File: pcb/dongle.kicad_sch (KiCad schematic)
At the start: 32 parts, among them J1 USB_A, J2 Conn_01x01_Pin, J3 Conn_01x01_Pin, J4 Conn_01x01_Pin, J5 Conn_01x01_Pin, SW1 SW_Push_45deg, U3 nRF52833_QDxx, Y1 32MHz

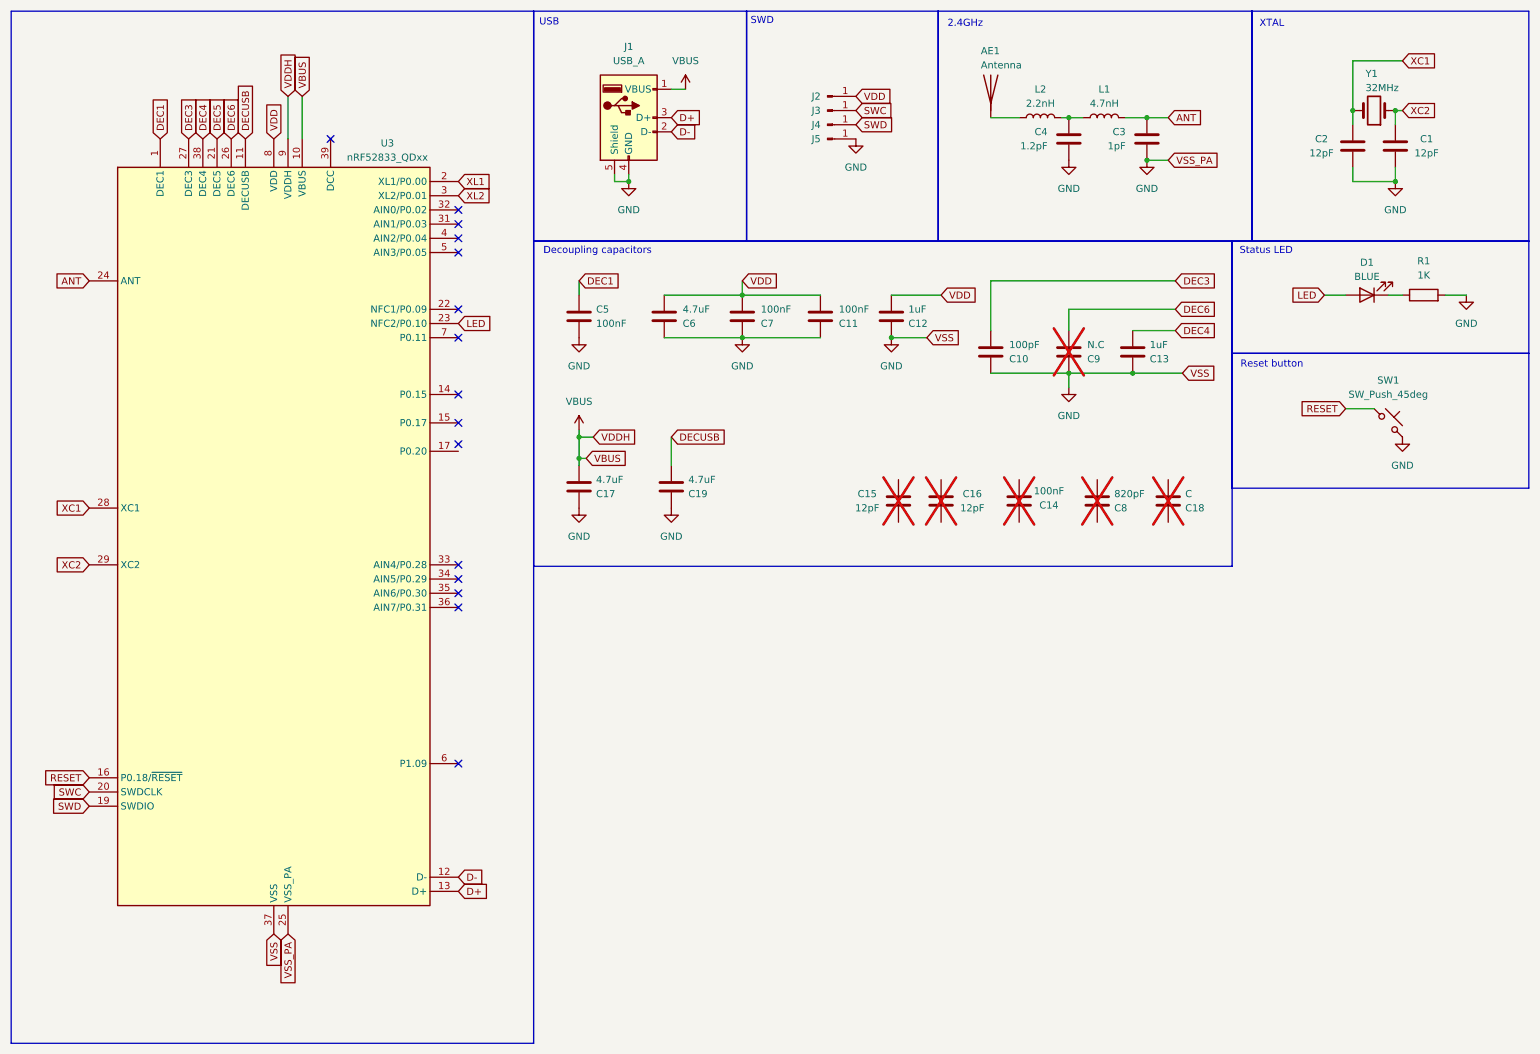
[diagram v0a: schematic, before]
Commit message: update pcb
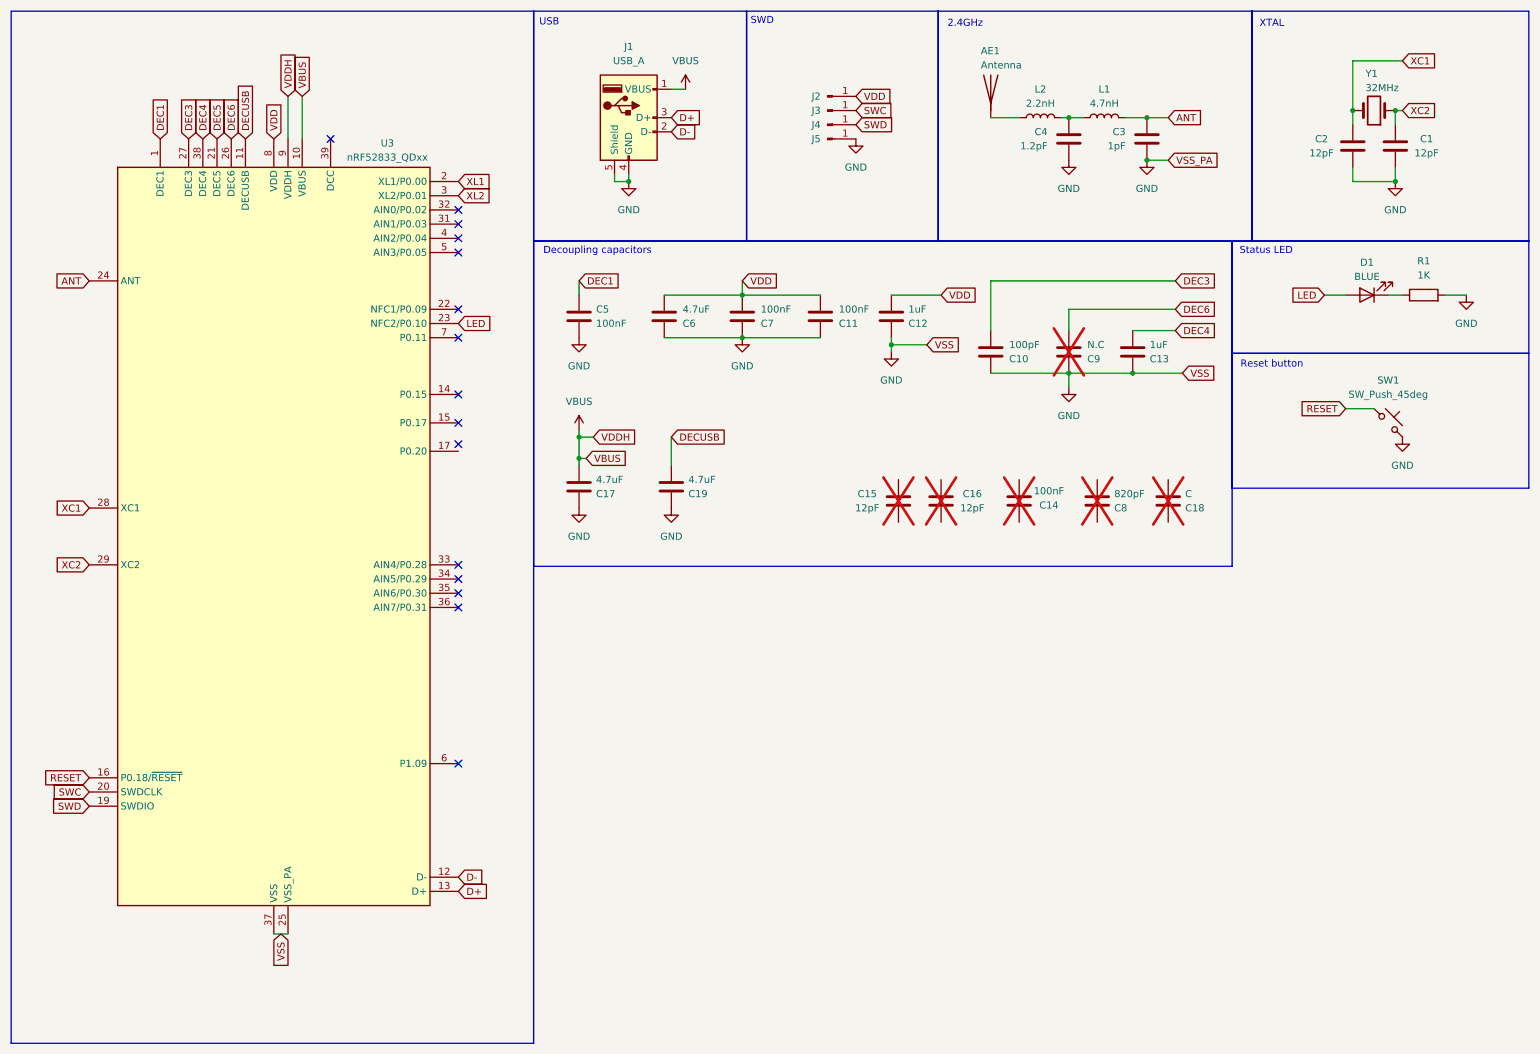
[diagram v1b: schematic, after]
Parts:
- AE1: footprint (none) -> dongle:Texas_SWRA117D_2.4GHz_Left
- D1: footprint (none) -> dongle:LED_0603_1608Metric
- R1: footprint (none) -> dongle:R_0201_0603Metric_Pad0.64x0.40mm_HandSolder
- SW1: footprint (none) -> dongle:TS342A2P
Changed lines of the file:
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@@
 	)
 	(junction
+		(at 170.18 72.39)
+		(diameter 0)
+		(color 0 0 0 0)
+	)
+	(junction
 		(at 201.93 31.75)
 		(diameter 0)
@@
 	)
 	(junction
-		(at 170.18 71.12)
-		(diameter 0)
-		(color 0 0 0 0)
-	)
-	(junction
 		(at 114.3 92.71)
 		(diameter 0)
@@
 	(wire
 		(pts
+			(xy 170.18 72.39) (xy 170.18 73.66)
+		)
+		(stroke
+			(width 0)
+			(type default)
+		)
+	)
+	(wire
+		(pts
 			(xy 220.98 60.96) (xy 187.96 60.96)
 		)
@@
 	(wire
 		(pts
+			(xy 170.18 71.12) (xy 170.18 72.39)
+		)
+		(stroke
+			(width 0)
+			(type default)
+		)
+	)
+	(wire
+		(pts
 			(xy 219.71 39.37) (xy 215.9 39.37)
 		)
@@
 	(wire
 		(pts
+			(xy 176.53 72.39) (xy 170.18 72.39)
+		)
+		(stroke
+			(width 0)
+			(type default)
+		)
+	)
+	(wire
+		(pts
 			(xy 251.46 63.5) (xy 247.65 63.5)
 		)
@@
 	(wire
 		(pts
-			(xy 273.05 63.5) (xy 269.24 63.5)
+			(xy 59.69 177.8) (xy 62.23 177.8)
 		)
 		(stroke
@@
 	(wire
 		(pts
-			(xy 252.73 21.59) (xy 252.73 30.48)
+			(xy 273.05 63.5) (xy 269.24 63.5)
 		)
 		(stroke
@@
 	(wire
 		(pts
-			(xy 176.53 71.12) (xy 170.18 71.12)
+			(xy 252.73 21.59) (xy 252.73 30.48)
 		)
 		(stroke
@@
 		)
 	)
-	(global_label "VSS"
+	(global_label "D+"
 		(shape input)
-		(at 176.53 71.12 0)
+		(at 130.81 31.75 0)
 		(fields_autoplaced yes)
 		(effects
@@
 		)
 		(property "Intersheetrefs" "${INTERSHEET_REFS}"
-			(at 183.0228 71.12 0)
+			(at 136.6376 31.75 0)
 			(effects
 				(font
@@
 		)
 	)
-	(global_label "D+"
+	(global_label "DEC5"
 		(shape input)
-		(at 130.81 31.75 0)
+		(at 49.53 35.56 90)
 		(fields_autoplaced yes)
 		(effects
@@
 		)
 		(property "Intersheetrefs" "${INTERSHEET_REFS}"
-			(at 136.6376 31.75 0)
+			(at 49.53 27.6763 90)
 			(effects
 				(font
@@
 		)
 	)
-	(global_label "DEC5"
+	(global_label "DEC1"
 		(shape input)
-		(at 49.53 35.56 90)
+		(at 39.37 35.56 90)
 		(fields_autoplaced yes)
 		(effects
@@
 		)
 		(property "Intersheetrefs" "${INTERSHEET_REFS}"
-			(at 49.53 27.6763 90)
+			(at 39.37 27.6763 90)
 			(effects
 				(font
@@
 		)
 	)
-	(global_label "DEC1"
+	(global_label "ANT"
 		(shape input)
-		(at 39.37 35.56 90)
+		(at 219.71 31.75 0)
 		(fields_autoplaced yes)
 		(effects
@@
 		)
 		(property "Intersheetrefs" "${INTERSHEET_REFS}"
-			(at 39.37 27.6763 90)
+			(at 226.0819 31.75 0)
 			(effects
 				(font
@@
 		)
 	)
-	(global_label "ANT"
+	(global_label "VDD"
 		(shape input)
-		(at 219.71 31.75 0)
+		(at 59.69 35.56 90)
 		(fields_autoplaced yes)
 		(effects
@@
 		)
 		(property "Intersheetrefs" "${INTERSHEET_REFS}"
-			(at 226.0819 31.75 0)
+			(at 59.69 28.9462 90)
 			(effects
 				(font
@@
 		)
 	)
-	(global_label "VDD"
+	(global_label "VSS"
 		(shape input)
-		(at 59.69 35.56 90)
+		(at 176.53 72.39 0)
 		(fields_autoplaced yes)
 		(effects
@@
 		)
 		(property "Intersheetrefs" "${INTERSHEET_REFS}"
-			(at 59.69 28.9462 90)
+			(at 183.0228 72.39 0)
 			(effects
 				(font
@@
 		)
 	)
-	(global_label "VSS"
-		(shape input)
-		(at 59.69 177.8 270)
-		(fields_autoplaced yes)
-		(effects
-			(font
-				(size 1.27 1.27)
-			)
-			(justify right)
-		)
-		(property "Intersheetrefs" "${INTERSHEET_REFS}"
-			(at 59.69 184.2928 90)
-			(effects
-				(font
-					(size 1.27 1.27)
-				)
-				(justify right)
-				(hide yes)
-			)
-		)
-	)
 	(global_label "DEC1"
 		(shape input)
@@
 		)
 	)
+	(global_label "VSS"
+		(shape input)
+		(at 60.96 177.8 270)
+		(fields_autoplaced yes)
+		(effects
+			(font
+				(size 1.27 1.27)
+			)
+			(justify right)
+		)
+		(property "Intersheetrefs" "${INTERSHEET_REFS}"
+			(at 60.96 184.2928 90)
+			(effects
+				(font
+					(size 1.27 1.27)
+				)
+				(justify right)
+				(hide yes)
+			)
+		)
+	)
 	(global_label "VDD"
 		(shape input)
@@
 		)
 	)
-	(global_label "VSS_PA"
-		(shape input)
-		(at 62.23 177.8 270)
-		(fields_autoplaced yes)
-		(effects
-			(font
-				(size 1.27 1.27)
-			)
-			(justify right)
-		)
-		(property "Intersheetrefs" "${INTERSHEET_REFS}"
-			(at 62.23 187.619 90)
-			(effects
-				(font
-					(size 1.27 1.27)
-				)
-				(justify right)
-				(hide yes)
-			)
-		)
-	)
 	(global_label "DEC6"
 		(shape input)
@@
 			)
 		)
-		(property "Footprint" ""
+		(property "Footprint" "dongle:TS342A2P"
 			(at 259.08 86.36 0)
 			(effects
@@
 	(symbol
 		(lib_id "Library:GND")
-		(at 170.18 71.12 0)
+		(at 170.18 73.66 0)
 		(unit 1)
 		(exclude_from_sim no)
@@
 		(fields_autoplaced yes)
 		(property "Reference" "#PWR07"
-			(at 170.18 77.47 0)
+			(at 170.18 80.01 0)
 			(effects
 				(font
@@
 		)
 		(property "Value" "GND"
-			(at 170.18 76.2 0)
+			(at 170.18 78.74 0)
 			(effects
 				(font
@@
 		)
 		(property "Footprint" ""
-			(at 170.18 71.12 0)
+			(at 170.18 73.66 0)
 			(effects
 				(font
@@
 		)
 		(property "Datasheet" ""
-			(at 170.18 71.12 0)
+			(at 170.18 73.66 0)
 			(effects
 				(font
@@
 		)
 		(property "Description" "Global ground symbol"
-			(at 170.18 80.518 0)
+			(at 170.18 83.058 0)
 			(effects
 				(font
@@
 			)
 		)
-		(property "Footprint" ""
+		(property "Footprint" "dongle:Texas_SWRA117D_2.4GHz_Left"
 			(at 187.96 26.67 0)
 			(effects
@@
 			)
 		)
-		(property "Footprint" ""
+		(property "Footprint" "dongle:R_0201_0603Metric_Pad0.64x0.40mm_HandSolder"
 			(at 265.43 65.278 90)
 			(effects
@@
 			)
 		)
-		(property "Footprint" ""
+		(property "Footprint" "dongle:LED_0603_1608Metric"
 			(at 255.27 63.5 0)
 			(effects

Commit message: update pcb
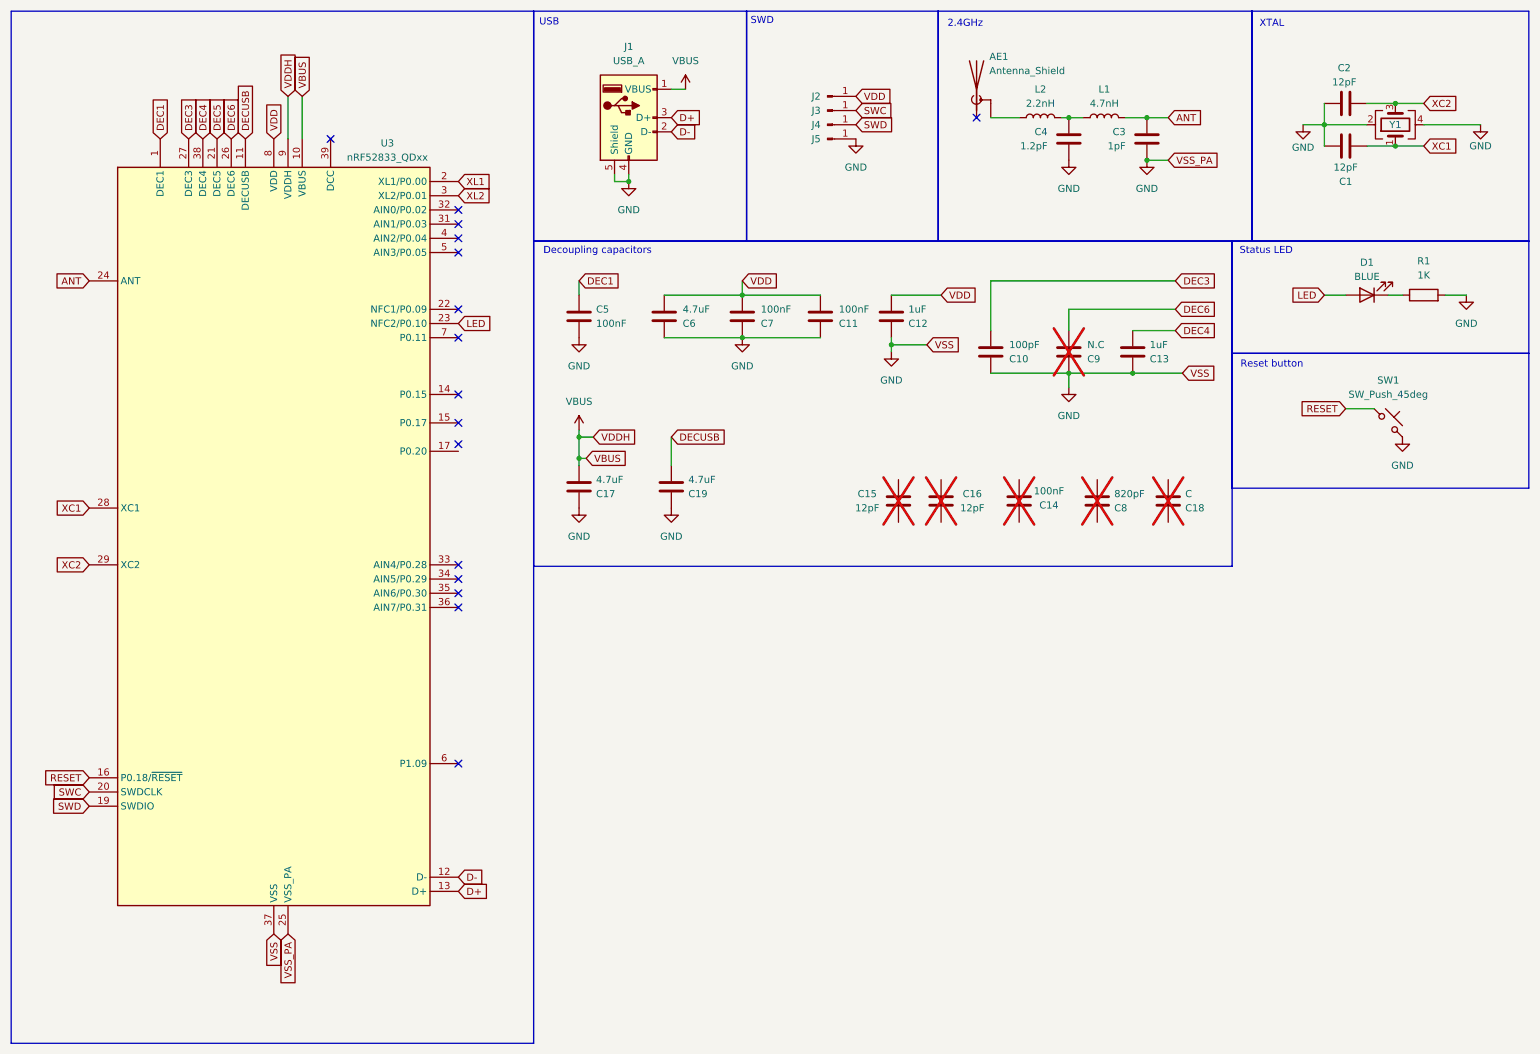
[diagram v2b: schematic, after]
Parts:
- removed AE1: Antenna, dongle:Texas_SWRA117D_2.4GHz_Left, symbol dongle:Antenna
- removed Y1: 32MHz, dongle:Crystal_SMD_2012-2Pin_2.0x1.2mm_HandSoldering, symbol PNCATEHO_lowair:Crystal
- added AE1: Antenna_Shield, dongle:ANTC5020X110N, symbol dongle:Antenna_Shield
- added Y1: Crystal_GND24, dongle:Crystal_SMD_3225-4Pin_3.2x2.5mm, symbol dongle:Crystal_GND24
- C1, C10, C11, C2, C3, C4, C5, C7: footprint dongle:C_0201_0603Metric_Pad0.64x0.40mm_HandSolder -> dongle:C_0201_0603Metric
- C12, C13: footprint dongle:C_0402_1005Metric_Pad0.74x0.62mm_HandSolder -> dongle:C_0402_1005Metric
- C17, C19, C6: footprint dongle:C_0603_1608Metric_Pad1.08x0.95mm_HandSolder -> dongle:C_0603_1608Metric
- D1: footprint dongle:LED_0603_1608Metric -> dongle:LED_0402_1005Metric
- J2, J3, J4: footprint dongle:TestPoint_Pad_1.0x1.0mm -> dongle:TestPoint_Pad_D1.0mm
- J5: footprint dongle:TestPoint_Pad_D1.0mm -> dongle:TestPoint_Pad_1.0x1.0mm
- L1, L2: footprint dongle:L_0201_0603Metric_Pad0.64x0.40mm_HandSolder -> dongle:L_0201_0603Metric
- R1: footprint dongle:R_0201_0603Metric_Pad0.64x0.40mm_HandSolder -> dongle:R_0402_1005Metric
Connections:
- net GND: now also C1.1, Y1.2, Y1.4; no longer C1.2
- net XC1: now also C1.2, Y1.1; no longer C2.2
- net XC2: now also C2.2, Y1.3; no longer C1.1
- net at L2.2: now also AE1.2 (Shield)
- no-connect marks 15 -> 16
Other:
- moved on the sheet: C1, C2
